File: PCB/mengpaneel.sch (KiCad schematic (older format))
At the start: 308 parts, among them IC1 MAX7219CNG+, IC10 STM32F411CEU7, IC11 AD5204BRUZ10-REEL7, IC13 LMV321AUIDBVR, IC2 MAX7219CNG+, IC3 MTCH6301-I_ML, IC5 AD5204BRUZ10-REEL7, IC6 AD5204BRUZ10-REEL7, IC8 AD5204BRUZ10-REEL7, IC9 AD5204BRUZ10-REEL7, J1 UJ2-MIBH-G-SMT-TR, J10 Screw_Terminal_01x01, J11 Screw_Terminal_01x01, J12 Screw_Terminal_01x01, J13 Screw_Terminal_01x01, J14 Screw_Terminal_01x01, J15 Screw_Terminal_01x01, J16 Screw_Terminal_01x01, J17 Screw_Terminal_01x01, J18 Screw_Terminal_01x12, J19 Screw_Terminal_01x05, J2 Screw_Terminal_01x01, J3 Screw_Terminal_01x14, J4 SJ-63053A, J5 SJ-63053A, J6 SJ-63053A, J7 SJ-63053A, J8 Screw_Terminal_01x01, J9 Screw_Terminal_01x01, SW1 SW_Push, SW2 SW_DPST_x2, SW3 SW_DPST_x2, SW4 SW_DPST_x2, U1 LM324A, U11 Touchpad_mp, U13 Touchpad_mp_LR, U14 Touchpad_mp, U15 Touchpad_mp, U16 Touchpad_mp, U17 Touchpad_mp, U2 Touchpad_mp, U3 Touchpad_mp, U4 Touchpad_mp, U5 LM324N, U6 Touchpad_mp, U7 LM324N, U8 Touchpad_mp, U9 LM324A, Y1 8MHz

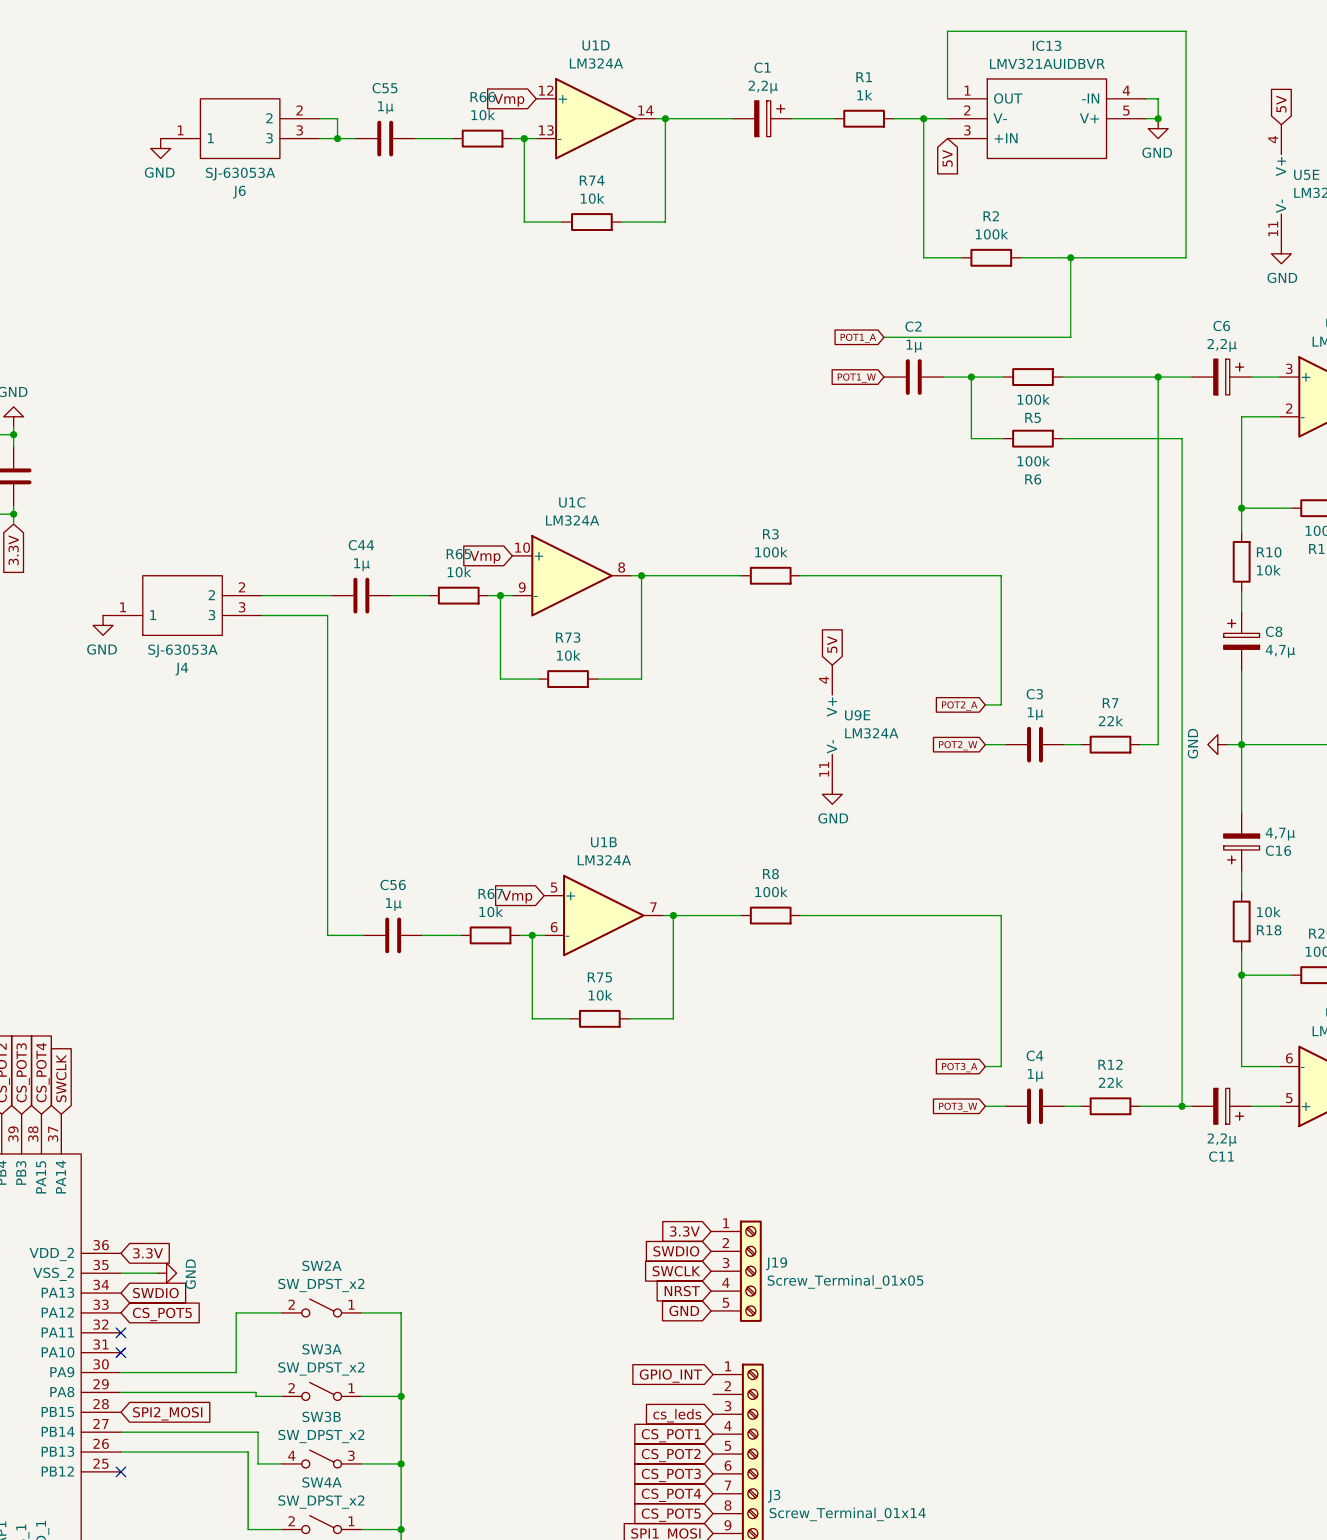
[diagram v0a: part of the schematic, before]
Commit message: Word document aangepast
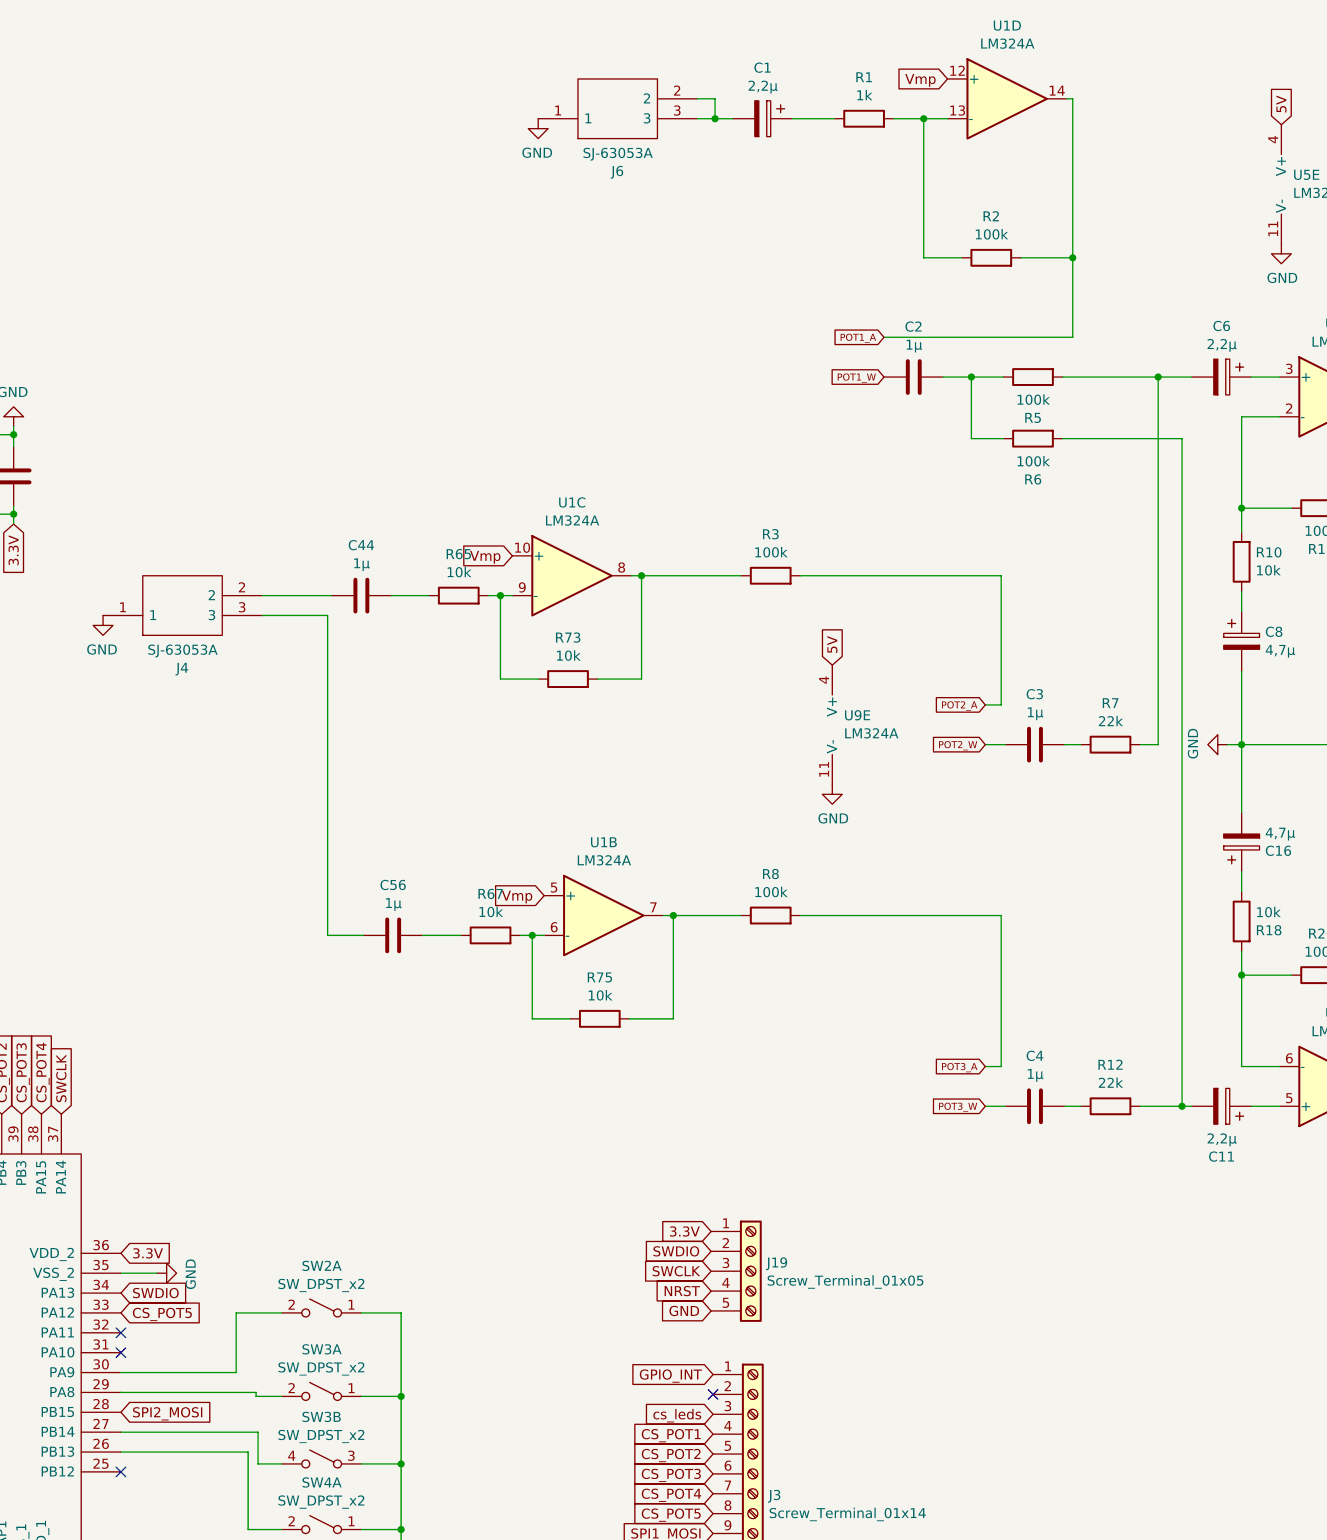
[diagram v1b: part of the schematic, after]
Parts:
- removed C55: 1µ, C0805X105K8RAC7210:CAPC2012X100N, symbol Device:C
- removed IC13: LMV321AUIDBVR, LMV321AUIDBVR:SOT95P280X145-5N, symbol LMV321AUIDBVR:LMV321AUIDBVR
- removed R66, R74: 10k, CMP2010-FX-1002ELF:RESC5025X70N, symbol Device:R
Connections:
- net POT1_A: now also U1.14
- net at R1.2, R2.1: now also U1.13 (-)
- net at C1.2: now also J6.2, J6.3; no longer U1.14
- no-connect marks 81 -> 82
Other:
- moved on the sheet: J6, U1D
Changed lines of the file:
@@
 	20820 4870 20960 4870
 Wire Wire Line
-	20520 4670 21460 4670
-Wire Wire Line
-	21460 4270 21460 4670
+	21470 4270 21470 4670
 $Comp
 L Device:CP C19
@@
 	20060 3570 20270 3570
 Wire Wire Line
-	21210 4270 21460 4270
-Wire Wire Line
 	20720 4270 20720 3570
 Wire Wire Line
@@
 L mengpaneel-rescue:SJ-63053A-SJ-63053A J6
 U 1 1 6D90AE19
-P 16880 3670
-F 0 "J6" H 17280 3935 50  0000 C CNN
-F 1 "SJ-63053A" H 17280 3844 50  0000 C CNN
-F 2 "SJ-63053A:SJ63053A" H 17530 3770 50  0001 L CNN
-F 3 "https://www.mouser.mx/datasheet/2/670/sj_63053a-1890674.pdf" H 17530 3670 50  0001 L CNN
-F 4 "Phone Connectors audio jack, 6.35 mm, horizontal, 3 conductor, through hole, 0 switches, w/ nut" H 17530 3570 50  0001 L CNN "Description"
-F 5 "12.8" H 17530 3470 50  0001 L CNN "Height"
-F 6 "490-SJ-63053A" H 17530 3370 50  0001 L CNN "Mouser Part Number"
-F 7 "https://www.mouser.co.uk/ProductDetail/CUI-Devices/SJ-63053A?qs=hWgE7mdIu5Q5ZZx8mXk5JQ%3D%3D" H 17530 3270 50  0001 L CNN "Mouser Price/Stock"
-F 8 "CUI Inc." H 17530 3170 50  0001 L CNN "Manufacturer_Name"
-F 9 "SJ-63053A" H 17530 3070 50  0001 L CNN "Manufacturer_Part_Number"
-	1    16880 3670
+P 18780 3570
+F 0 "J6" H 19180 3835 50  0000 C CNN
+F 1 "SJ-63053A" H 19180 3744 50  0000 C CNN
+F 2 "SJ-63053A:SJ63053A" H 19430 3670 50  0001 L CNN
+F 3 "https://www.mouser.mx/datasheet/2/670/sj_63053a-1890674.pdf" H 19430 3570 50  0001 L CNN
+F 4 "Phone Connectors audio jack, 6.35 mm, horizontal, 3 conductor, through hole, 0 switches, w/ nut" H 19430 3470 50  0001 L CNN "Description"
+F 5 "12.8" H 19430 3370 50  0001 L CNN "Height"
+F 6 "490-SJ-63053A" H 19430 3270 50  0001 L CNN "Mouser Part Number"
+F 7 "https://www.mouser.co.uk/ProductDetail/CUI-Devices/SJ-63053A?qs=hWgE7mdIu5Q5ZZx8mXk5JQ%3D%3D" H 19430 3170 50  0001 L CNN "Mouser Price/Stock"
+F 8 "CUI Inc." H 19430 3070 50  0001 L CNN "Manufacturer_Name"
+F 9 "SJ-63053A" H 19430 2970 50  0001 L CNN "Manufacturer_Part_Number"
+	1    18780 3570
 	1    0    0    1
 $EndComp
@@
 L power:GND #PWR0194
 U 1 1 6D90AE1F
-P 16880 3670
-F 0 "#PWR0194" H 16880 3420 50  0001 C CNN
-F 1 "GND" H 16885 3497 50  0000 C CNN
-F 2 "" H 16880 3670 50  0001 C CNN
-F 3 "" H 16880 3670 50  0001 C CNN
-	1    16880 3670
+P 18780 3570
+F 0 "#PWR0194" H 18780 3320 50  0001 C CNN
+F 1 "GND" H 18785 3397 50  0000 C CNN
+F 2 "" H 18780 3570 50  0001 C CNN
+F 3 "" H 18780 3570 50  0001 C CNN
+	1    18780 3570
 	-1   0    0    -1
 $EndComp
@@
 Connection ~ 26140 18220
 Connection ~ 20720 3570
-Wire Wire Line
-	20840 3470 20840 3130
-Wire Wire Line
-	20840 3130 22040 3130
-Wire Wire Line
-	22040 3130 22040 4270
-Wire Wire Line
-	22040 4270 21460 4270
-Connection ~ 21460 4270
 Wire Notes Line
 	10260 12640 10260 18730
@@
 Text GLabel 22520 3600 1    50   Input ~ 0
 5V
-Text GLabel 20840 3670 3    50   Input ~ 0
-5V
-Wire Wire Line
-	21840 3570 21900 3570
-$Comp
-L LMV321AUIDBVR:LMV321AUIDBVR IC13
-U 1 1 64D50D66
-P 20840 3470
-F 0 "IC13" H 21340 3735 50  0000 C CNN
-F 1 "LMV321AUIDBVR" H 21340 3644 50  0000 C CNN
-F 2 "LMV321AUIDBVR:SOT95P280X145-5N" H 21690 3570 50  0001 L CNN
-F 3 "https://www.ti.com/lit/gpn/LMV321A" H 21690 3470 50  0001 L CNN
-F 4 "Operational Amplifiers - Op Amps Single Low-Voltage, Cost-Optimized Rail-to-Rail Output Operational Amplifier 5-SOT-23 -40 to 125" H 21690 3370 50  0001 L CNN "Description"
-F 5 "1.45" H 21690 3270 50  0001 L CNN "Height"
-F 6 "595-LMV321AUIDBVR" H 21690 3170 50  0001 L CNN "Mouser Part Number"
-F 7 "https://www.mouser.co.uk/ProductDetail/Texas-Instruments/LMV321AUIDBVR/?qs=GBLSl2AkirulEcoP6K7rtg%3D%3D" H 21690 3070 50  0001 L CNN "Mouser Price/Stock"
-F 8 "Texas Instruments" H 21690 2970 50  0001 L CNN "Manufacturer_Name"
-F 9 "LMV321AUIDBVR" H 21690 2870 50  0001 L CNN "Manufacturer_Part_Number"
-	1    20840 3470
-	1    0    0    -1
-$EndComp
 Wire Wire Line
 	20720 3570 20840 3570
-Wire Wire Line
-	21840 3470 21900 3470
-Wire Wire Line
-	21900 3470 21900 3570
-$Comp
-L power:GND #PWR0104
-U 1 1 5FAA7B85
-P 21900 3570
-F 0 "#PWR0104" H 21900 3320 50  0001 C CNN
-F 1 "GND" H 21905 3397 50  0000 C CNN
-F 2 "" H 21900 3570 50  0001 C CNN
-F 3 "" H 21900 3570 50  0001 C CNN
-	1    21900 3570
-	-1   0    0    -1
-$EndComp
-Connection ~ 21900 3570
 Text GLabel 15550 12900 1    50   Input ~ 0
 5V
@@
 Wire Wire Line
 	17720 6070 17390 6070
-Wire Wire Line
-	19420 4090 19420 3570
-Wire Wire Line
-	19420 3570 19370 3570
-Text GLabel 18770 3470 0    50   Input ~ 0
+Text GLabel 20840 3370 0    50   Input ~ 0
 Vmp
 Wire Wire Line
-	18160 3670 18350 3670
-Wire Wire Line
-	19200 4090 19420 4090
+	19580 3570 19670 3570
 Wire Wire Line
-	18710 3670 18770 3670
-Connection ~ 18710 3670
+	19580 3470 19670 3470
 Wire Wire Line
-	18650 3670 18710 3670
+	19670 3470 19670 3570
+Connection ~ 19670 3570
 Wire Wire Line
-	18710 4090 18900 4090
-Wire Wire Line
-	18710 3670 18710 4090
-$Comp
-L Device:R R74
-U 1 1 6D09B198
-P 19050 4090
-F 0 "R74" V 19257 4090 50  0000 C CNN
-F 1 "10k" V 19166 4090 50  0000 C CNN
-F 2 "CMP2010-FX-1002ELF:RESC5025X70N" V 18980 4090 50  0001 C CNN
-F 3 "~" H 19050 4090 50  0001 C CNN
-	1    19050 4090
-	0    -1   -1   0
-$EndComp
-$Comp
-L Device:R R66
-U 1 1 6D09B19E
-P 18500 3670
-F 0 "R66" V 18707 3670 50  0000 C CNN
-F 1 "10k" V 18616 3670 50  0000 C CNN
-F 2 "CMP2010-FX-1002ELF:RESC5025X70N" V 18430 3670 50  0001 C CNN
-F 3 "~" H 18500 3670 50  0001 C CNN
-	1    18500 3670
-	0    -1   -1   0
-$EndComp
-$Comp
-L Device:C C55
-U 1 1 6D09B1A4
-P 18010 3670
-F 0 "C55" V 18262 3670 50  0000 C CNN
-F 1 "1µ" V 18171 3670 50  0000 C CNN
-F 2 "C0805X105K8RAC7210:CAPC2012X100N" H 18048 3520 50  0001 C CNN
-F 3 "~" H 18010 3670 50  0001 C CNN
-	1    18010 3670
-	0    -1   -1   0
-$EndComp
-Wire Wire Line
-	19420 3570 19760 3570
-Connection ~ 19420 3570
-Wire Wire Line
-	17680 3670 17770 3670
-Wire Wire Line
-	17680 3570 17770 3570
-Wire Wire Line
-	17770 3570 17770 3670
-Connection ~ 17770 3670
-Wire Wire Line
-	17770 3670 17860 3670
+	19670 3570 19760 3570
 $Comp
 L Amplifier_Operational:LM324A U1
 U 4 1 6D81755F
-P 19070 3570
-F 0 "U1" H 19070 3937 50  0000 C CNN
-F 1 "LM324A" H 19070 3846 50  0000 C CNN
-F 2 "LM324N:DIP794W56P254L1905H533Q14N" H 19020 3670 50  0001 C CNN
-F 3 "http://www.ti.com/lit/ds/symlink/lm2902-n.pdf" H 19120 3770 50  0001 C CNN
-	4    19070 3570
+P 21140 3470
+F 0 "U1" H 21140 3837 50  0000 C CNN
+F 1 "LM324A" H 21140 3746 50  0000 C CNN
+F 2 "LM324N:DIP794W56P254L1905H533Q14N" H 21090 3570 50  0001 C CNN
+F 3 "http://www.ti.com/lit/ds/symlink/lm2902-n.pdf" H 21190 3670 50  0001 C CNN
+	4    21140 3470
 	1    0    0    -1
 $EndComp
@@
 NoConn ~ 12280 13380
 NoConn ~ 15780 11080
+Wire Wire Line
+	21440 3470 21470 3470
+Wire Wire Line
+	21470 3470 21470 4270
+Wire Wire Line
+	21210 4270 21470 4270
+Connection ~ 21470 4270
+Wire Wire Line
+	20520 4670 21470 4670
+NoConn ~ 19660 9990
 $EndSCHEMATC
